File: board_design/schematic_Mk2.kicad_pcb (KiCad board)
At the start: 2 copper layers, 88 x 68 mm, 29 parts, among them J1 A-DF_09_A_KG-T4S, J2 1757255, SW1 On/Off Switch, U1 ESP32-DEVKITC-32D, U2 LTV-846S

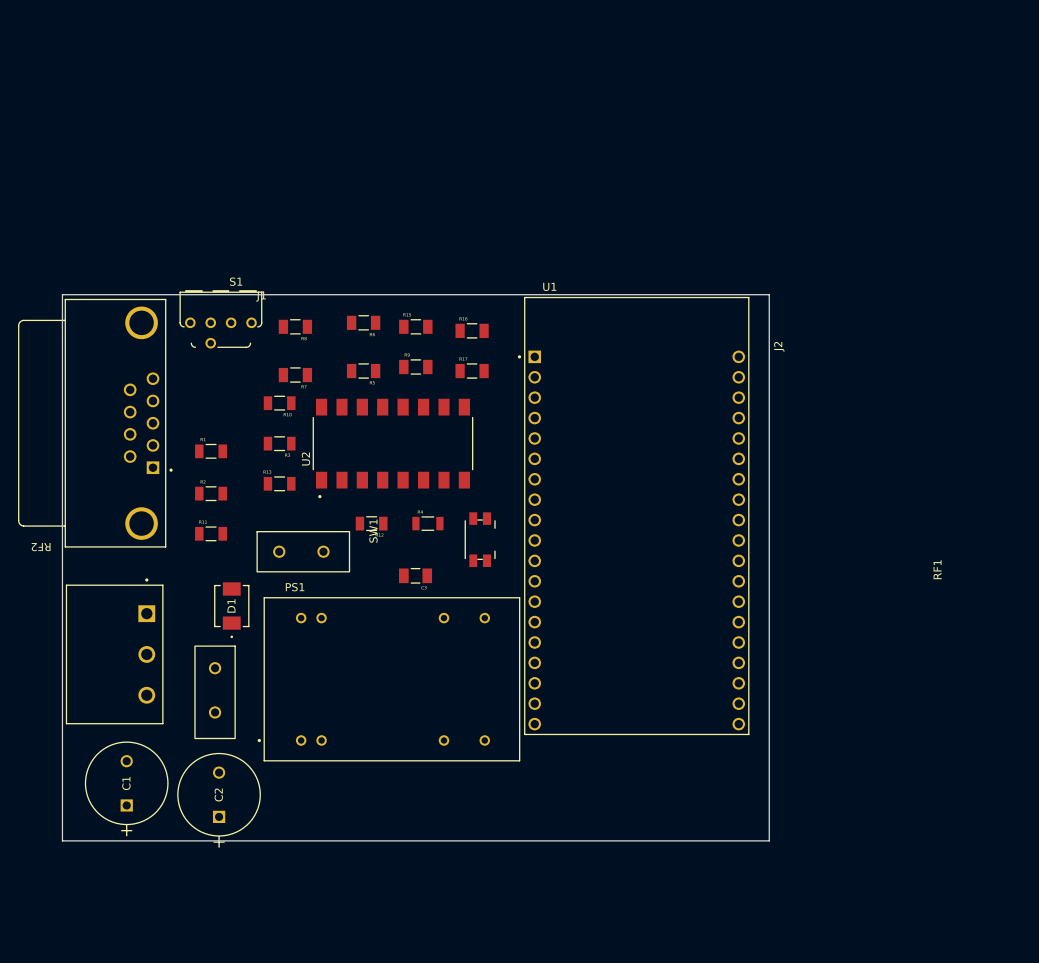
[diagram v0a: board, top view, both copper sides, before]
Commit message: updating board
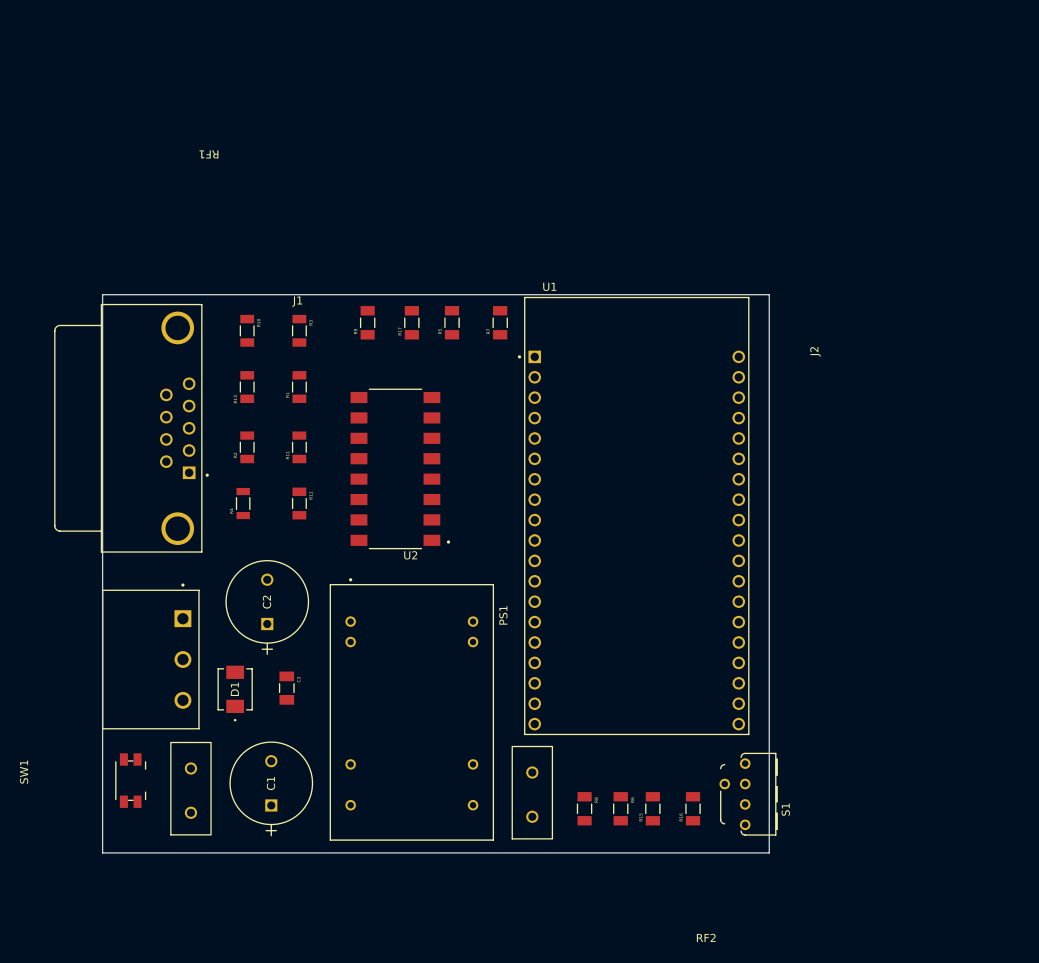
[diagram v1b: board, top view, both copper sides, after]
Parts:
- moved S1 87.8 mm to (201.5, 93.7), turned to 90 degrees
- moved R8 70.0 mm to (181.5, 95.5), turned to -90 degrees
- moved R6 68.4 mm to (186.0, 95.5), turned to -90 degrees
- moved R15 66.9 mm to (190.0, 95.5), turned to 90 degrees
- moved R16 65.6 mm to (195.0, 95.5), turned to 90 degrees
- moved SW1 52.8 mm to (125.0, 92.0)
- moved RF2 43.6 mm to (175.0, 96.5), turned to 90 degrees
- moved RF1 34.3 mm to (132.5, 96.0), turned to 90 degrees
- moved R7 26.3 mm to (171.0, 35.0), turned to 90 degrees
- moved C2 24.8 mm to (142.0, 72.5)
- moved R4 23.1 mm to (139.0, 57.5), turned to 90 degrees
- moved C3 21.3 mm to (144.4, 80.5), turned to -90 degrees
- moved C1 18.0 mm to (142.5, 95.1)
- moved R11 15.4 mm to (146.0, 50.5), turned to 90 degrees
- moved R3 14.3 mm to (146.0, 36.0), turned to -90 degrees
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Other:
- board size 88 x 68 mm -> 83 x 69.5 mm

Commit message: pcb update
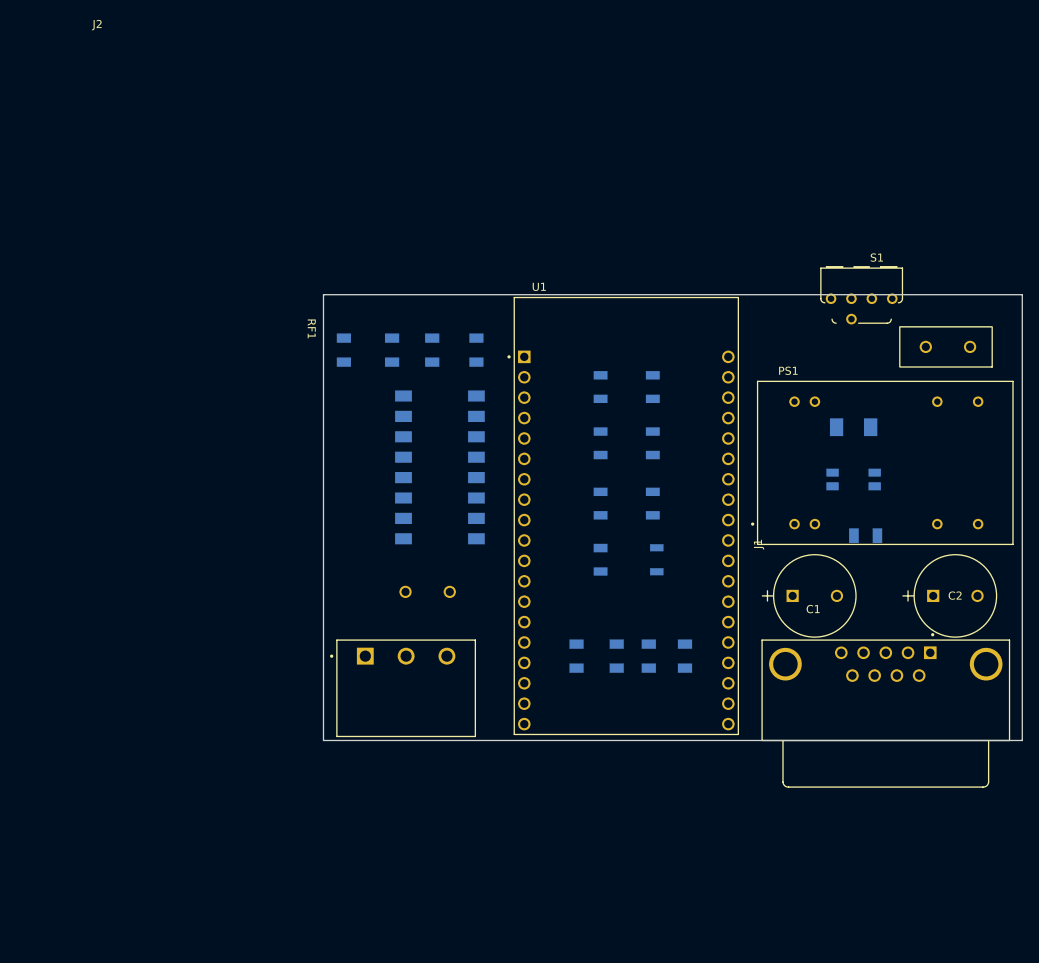
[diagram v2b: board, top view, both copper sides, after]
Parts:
- C3, D1, R1, R10, R11, R12, R13, R15, R16, R17, R2, R3, R4, R5, R6, R7, R8, R9, RF2, SW1, U2: moved to B.Cu
- moved RF1 113.0 mm to (229.5, 38.0), turned to 180 degrees
- moved SW1 97.5 mm to (215.0, 54.5), turned to 0 degrees
- moved J1 95.0 mm to (224.5, 76.1), turned to 0 degrees
- moved D1 83.6 mm to (215.0, 48.0), turned to 0 degrees
- moved C2 83.0 mm to (224.9, 69.0), turned to 0 degrees
- moved C3 74.5 mm to (216.5, 61.5), turned to 0 degrees
- moved C1 70.0 mm to (207.4, 69.0), turned to 0 degrees
- moved PS1 66.6 mm to (218.9, 52.4), turned to 0 degrees
- moved S1 63.4 mm to (216.0, 32.0), turned to 180 degrees
- moved R4 52.0 mm to (190.5, 64.5)
- moved R10 51.0 mm to (190.0, 43.0)
- moved R13 51.0 mm to (190.0, 50.0)
- moved R2 51.0 mm to (190.0, 57.5)
- moved R1 38.1 mm to (183.5, 50.0)
- moved R11 38.1 mm to (183.5, 57.5)
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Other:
- board size 83 x 69.5 mm -> 87 x 55.5 mm
